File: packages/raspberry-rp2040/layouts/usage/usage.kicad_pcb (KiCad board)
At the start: 4 copper layers, 36 parts

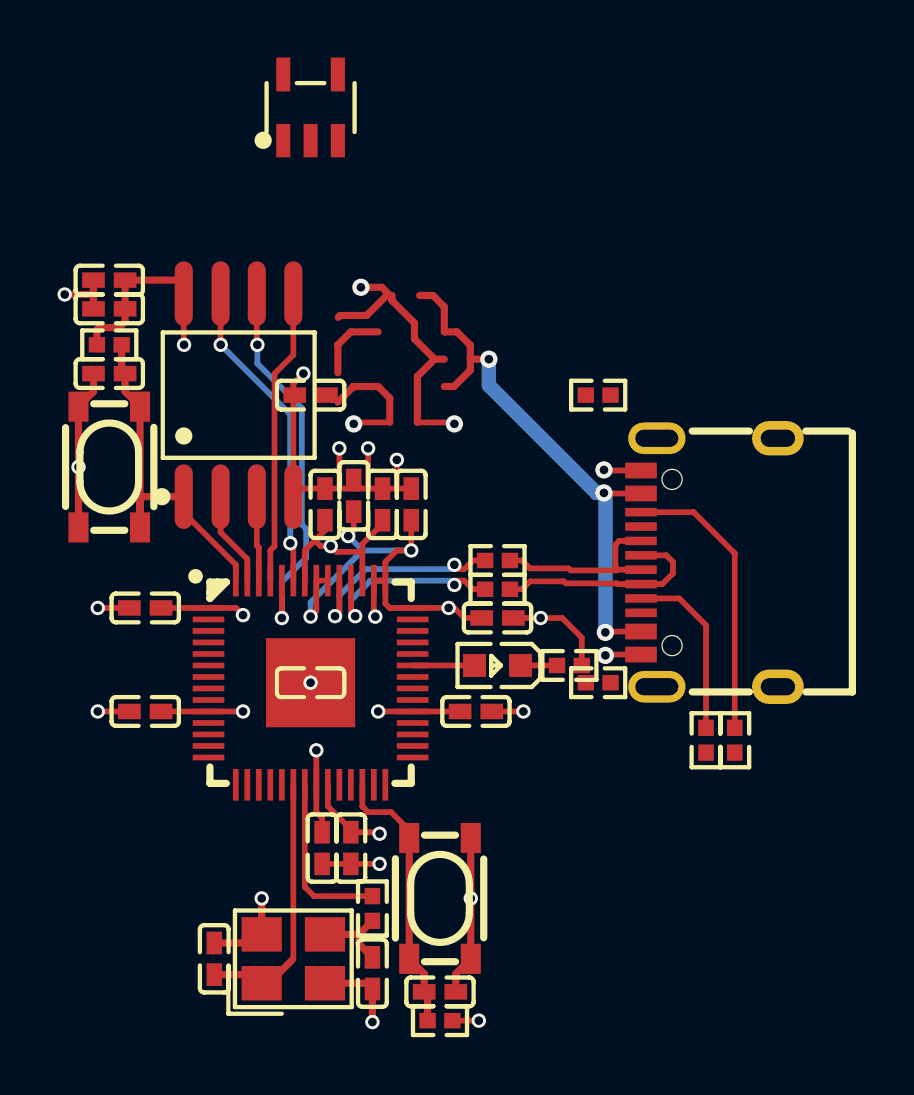
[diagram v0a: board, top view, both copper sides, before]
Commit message: update usage
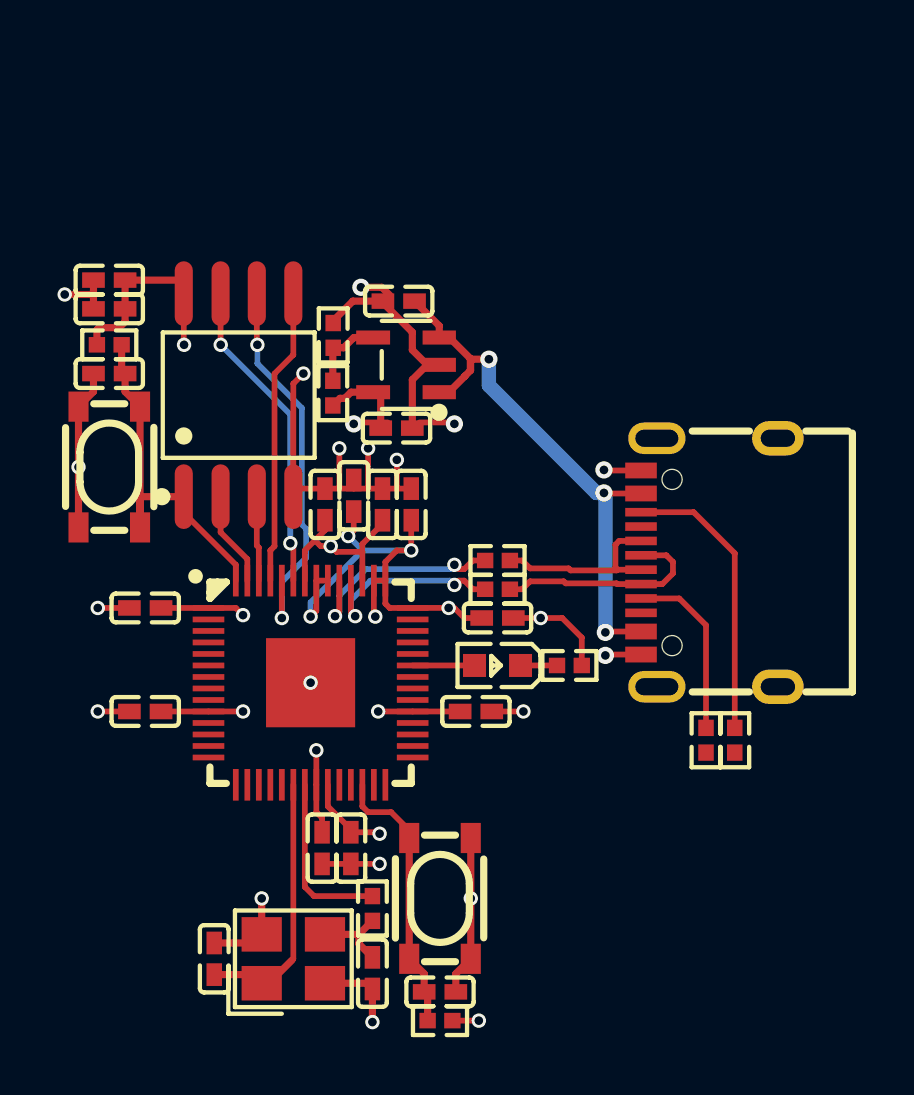
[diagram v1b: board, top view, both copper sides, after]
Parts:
- R1: value 10kΩ ±1% 62.5mW -> 5.1kΩ ±1% 62.5mW; footprint UNI_ROYAL_0402WGF1002TCE:R0402 -> UNI_ROYAL_0402WGF5101TCE:R0402
- R2: value 20kΩ ±1% 62.5mW -> 10kΩ ±1% 62.5mW; footprint UNI_ROYAL_0402WGF2002TCE:R0402 -> UNI_ROYAL_0402WGF1002TCE:R0402
- R7, R8: footprint YAGEO_RC0402FR_0727RL:R0402 -> UNI_ROYAL_0402WGF270JTCE:R0402
- moved R1 15.2 mm to (0.79, -12.1), turned to 90 degrees
- moved C1 13.6 mm to (3.06, -13.3), turned to 180 degrees
- moved U1 9.54 mm to (3.32, -11.1), turned to 90 degrees
- moved R2 9.23 mm to (0.77, -10.1), turned to 90 degrees
- moved C2 3.20 mm to (2.99, -8.85)
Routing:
- net (no net): track 22.1 -> 0.00 mm, vias 3 -> 0
- net hv: track 0.00 -> 19.7 mm, vias 0 -> 3
- net ADJ_NC: track 0.00 -> 2.69 mm
